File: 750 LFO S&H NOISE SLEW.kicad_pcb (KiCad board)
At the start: 2 copper layers, 65 x 106.5 mm, 239 parts, among them J1 PJ301BM, J10 PJ301BM, J11 PJ301BM, J2 PJ301BM, J3 PJ301BM, J4 PJ301BM, J5 JACK_MONO_SW, J6 PJ301BM, J7 JACK_MONO_SW, J8 PJ301BM, J9 PJ301BM, P1 CONN_01X03, P3 CONN_02X05, Q1 MMBT3904, Q10 MMBT3904, Q11 J112, Q12 MMBT3906, Q13 J112, Q14 J112, Q15 MMBT3904, Q16 MMBT3904, Q2 MMBT3904, Q3 2N7002, Q4 2N7002, Q5 MBT3946DW, Q6 MBT3946DW, Q7 MMBT3904, Q8 MMBT3904, Q9 MMBT3904, SW1 KS-01Q, SW2 KS-01Q, SW3 SPDT, U1 LM13700, U10 TL072-, U11 TL072-, U12 MAX9945, U13 DG409, U14 DG409, U15 TS321, U2 TL072-, U3 TL072-, U4 TL072-, U5 TL072-, U6 CD40106, U7 CD4027, U8 CD4027, U9 TL072-

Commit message: notes
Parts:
- R25: value 10K -> 22K
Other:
- board text removed: "SN#"
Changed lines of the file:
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@@
     (links 501)
     (no_connects 0)
-    (area 59.924999 24.924999 125.075001 131.575001)
+    (area 56.936905 22.45604 128.313095 132.325001)
     (thickness 1.6)
     (drawings 942)
@@
     (35 F.Paste user)
     (36 B.SilkS user)
-    (37 F.SilkS user)
+    (37 F.SilkS user hide)
     (38 B.Mask user)
     (39 F.Mask user)
@@
     (pad_to_mask_clearance 0.01)
     (aux_axis_origin 0 0)
-    (visible_elements 7FFFF77F)
+    (visible_elements 7FFFB7FF)
     (pcbplotparams
       (layerselection 0x010f0_80000001)
@@
       (effects (font (size 0.6096 0.6096) (thickness 0.1524)) (justify mirror))
     )
-    (fp_text value 2N7002 (at 1.016 -2.286 90) (layer B.SilkS) hide
+    (fp_text value 2N7002 (at -1.25 -0.5 90) (layer B.SilkS) hide
       (effects (font (size 0.8128 0.8128) (thickness 0.1524)) (justify mirror))
     )
@@
       (effects (font (size 0.6096 0.6096) (thickness 0.1524)) (justify mirror))
     )
-    (fp_text value 2N7002 (at 1.016 -2.286 90) (layer B.SilkS) hide
+    (fp_text value 2N7002 (at 1.2 0.05 90) (layer B.SilkS) hide
       (effects (font (size 0.8128 0.8128) (thickness 0.1524)) (justify mirror))
     )
@@
       (effects (font (size 0.6096 0.6096) (thickness 0.1524)) (justify mirror))
     )
-    (fp_text value 1N4148 (at 0 -1.905 90) (layer B.SilkS) hide
+    (fp_text value 1N4148 (at 0.15 -0.05 90) (layer B.SilkS) hide
       (effects (font (size 1 1) (thickness 0.15)) (justify mirror))
     )
@@
       (effects (font (size 0.6096 0.6096) (thickness 0.1524)) (justify mirror))
     )
-    (fp_text value 10K (at 0 0 270) (layer B.SilkS) hide
+    (fp_text value 22K (at 0 0 270) (layer B.SilkS) hide
       (effects (font (size 0.508 0.4572) (thickness 0.1143)) (justify mirror))
     )
@@
     (at 75.5 45.5 180)
     (attr smd)
-    (fp_text reference R99 (at -3 -0.75 180) (layer B.SilkS)
+    (fp_text reference R99 (at -0.1 -1.4 180) (layer B.SilkS)
       (effects (font (size 0.6096 0.6096) (thickness 0.1524)) (justify mirror))
     )
@@
     )
   )
-  (gr_text SN# (at 113.5 129.9) (layer B.SilkS)
-    (effects (font (size 1 1) (thickness 0.15)) (justify mirror))
-  )
+  (gr_line (start 63.45 66.9) (end 63.45 66.9) (angle 90) (layer B.SilkS) (width 5))
   (gr_line (start 109.4 128.3) (end 106.4 128.3) (angle 90) (layer B.SilkS) (width 5))
   (gr_text 850 (at 92.4 128.4) (layer B.SilkS)
@@
   (gr_line (start 68.000117 32.50286) (end 68.000117 34.50286) (layer Eco2.User) (width 0.1))
   (gr_text -12V (at 116.1 111.7) (layer B.SilkS)
-    (effects (font (size 1 1) (thickness 0.1524)) (justify mirror))
+    (effects (font (size 1.2 1.2) (thickness 0.25)) (justify mirror))
   )
   (gr_line (start 123.75 109.75) (end 116.25 109.75) (angle 90) (layer B.SilkS) (width 2))

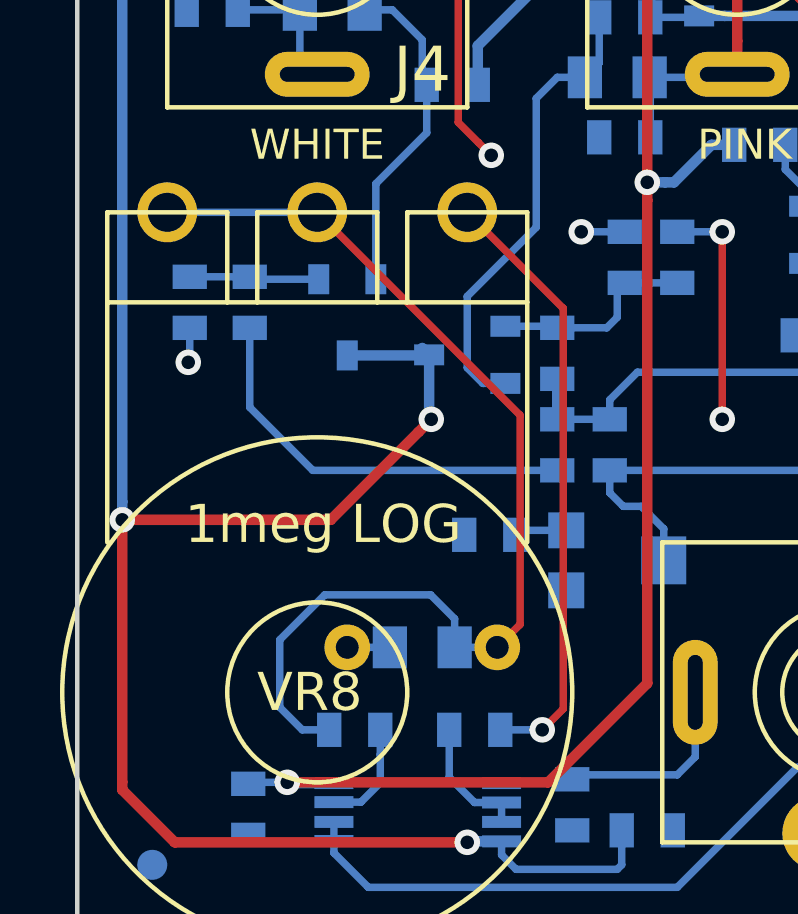
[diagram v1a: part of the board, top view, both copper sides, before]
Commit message: commit before adding voltage referencd for LFO
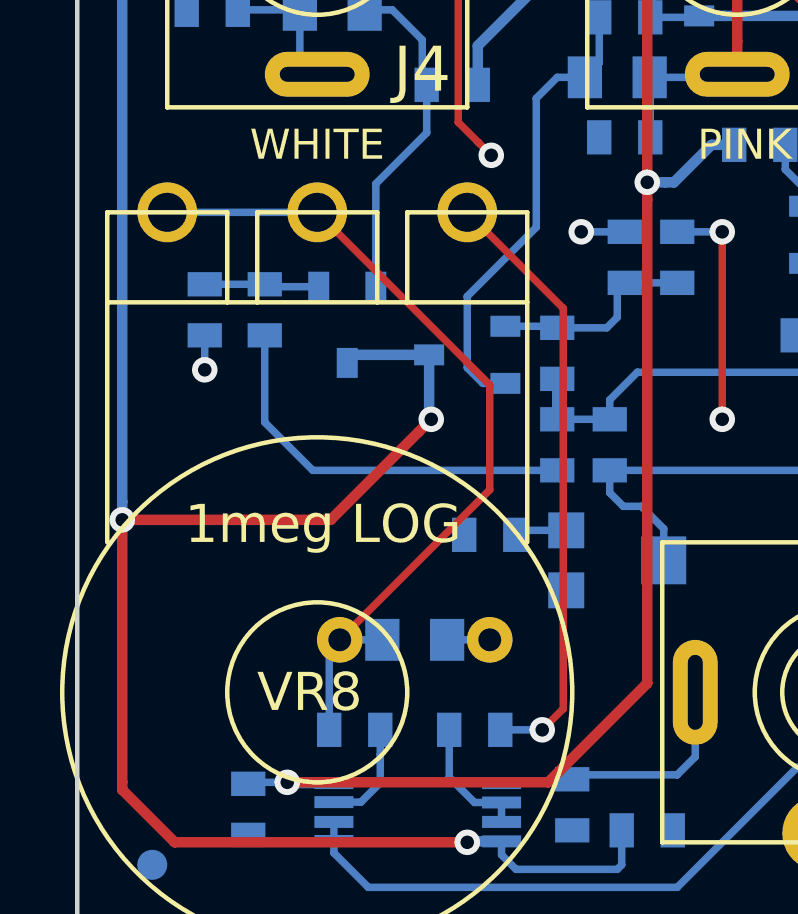
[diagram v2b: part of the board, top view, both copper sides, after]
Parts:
- moved R26 0.56 mm to (66.2, 110.8)
- moved R29 0.56 mm to (64.2, 110.8)
- moved C44 0.35 mm to (71.2, 121.8), turned to 0 degrees
- moved Q9 0.25 mm to (69.0, 111.2)
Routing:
- net Net-(C44-Pad1): track 36.0 -> 28.3 mm
- net Net-(Q9-Pad1): track 4.57 -> 4.07 mm
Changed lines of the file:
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@@
     (thickness 1.6)
     (drawings 942)
-    (tracks 1971)
+    (tracks 1964)
     (zones 0)
     (modules 239)
@@
   )
   (module MyModules:SOT23-132-JRL (layer B.Cu)
-    (at 69 111)
+    (at 69 111.25)
     (tags SOT23)
     (fp_text reference Q9 (at 1.99898 0.09906 270) (layer B.SilkS)
@@
   )
   (module MyModules:SM0603-R-JRL (layer B.Cu)
-    (at 65.75 110.5 90)
+    (at 66.25 110.75 90)
     (attr smd)
     (fp_text reference R26 (at 2 0 180) (layer B.SilkS)
@@
   )
   (module MyModules:SM0603-R-JRL (layer B.Cu)
-    (at 63.75 110.5 270)
+    (at 64.25 110.75 270)
     (attr smd)
     (fp_text reference R29 (at 0 1.4 270) (layer B.SilkS)
@@
   )
   (module MyModules:CAP-5MM-BOX-0805-COMBO (layer B.Cu)
-    (at 71.5 122 180)
-    (fp_text reference C44 (at 4.4 0 270) (layer B.SilkS)
+    (at 71.25 121.75)
+    (fp_text reference C44 (at 4.4 0 90) (layer B.SilkS)
       (effects (font (size 0.8128 0.8128) (thickness 0.1524)) (justify mirror))
     )
-    (fp_text value 470n (at 1.6 2.6 180) (layer B.Fab) hide
+    (fp_text value 470n (at 1.6 2.6) (layer B.Fab) hide
       (effects (font (size 1 1) (thickness 0.15)) (justify mirror))
     )
@@
     (fp_line (start -1.75 0.75) (end -1.75 -0.75) (layer B.SilkS) (width 0.15))
     (fp_line (start 1.75 0.75) (end 1.75 -0.75) (layer B.SilkS) (width 0.15))
-    (pad 1 thru_hole circle (at -2.5 0 180) (size 1.524 1.524) (drill 0.762) (layers *.Cu *.Mask B.SilkS)
+    (pad 1 thru_hole circle (at -2.5 0) (size 1.524 1.524) (drill 0.762) (layers *.Cu *.Mask B.SilkS)
       (net 35 "Net-(C44-Pad1)"))
-    (pad 2 thru_hole circle (at 2.5 0 180) (size 1.524 1.524) (drill 0.762) (layers *.Cu *.Mask B.SilkS)
+    (pad 2 thru_hole circle (at 2.5 0) (size 1.524 1.524) (drill 0.762) (layers *.Cu *.Mask B.SilkS)
       (net 1 GND))
-    (pad 1 smd rect (at -1.0795 0 180) (size 1.143 1.397) (layers B.Cu B.Paste B.Mask)
+    (pad 1 smd rect (at -1.0795 0) (size 1.143 1.397) (layers B.Cu B.Paste B.Mask)
       (net 35 "Net-(C44-Pad1)"))
-    (pad 2 smd rect (at 1.0795 0 180) (size 1.143 1.397) (layers B.Cu B.Paste B.Mask)
+    (pad 2 smd rect (at 1.0795 0) (size 1.143 1.397) (layers B.Cu B.Paste B.Mask)
       (net 1 GND))
   )
@@
   (gr_line (start 125 25) (end 125 131.5) (angle 90) (layer Edge.Cuts) (width 0.15))
   (gr_line (start 60 25) (end 125 25) (angle 90) (layer Edge.Cuts) (width 0.15))
+  (segment (start 64.25 111.6009) (end 64.25 112.75) (width 0.25) (layer B.Cu) (net 1))
+  (via (at 64.25 112.75) (size 0.85) (drill 0.45) (layers F.Cu B.Cu) (net 1))
+  (segment (start 72.3295 121.75) (end 73.75 121.75) (width 0.25) (layer B.Cu) (net 1))
   (segment (start 93.5 117.3) (end 90.7 114.5) (width 0.25) (layer F.Cu) (net 1))
   (segment (start 90.7 114.5) (end 90.1 114.5) (width 0.25) (layer F.Cu) (net 1))
@@
   (segment (start 96.1509 115.6509) (end 95.4 114.9) (width 0.25) (layer B.Cu) (net 1))
   (via (at 95.4 114.9) (size 0.85) (drill 0.45) (layers F.Cu B.Cu) (net 1))
-  (segment (start 63.75 111.3509) (end 63.75 112.45) (width 0.25) (layer B.Cu) (net 1))
-  (segment (start 63.75 112.45) (end 63.7 112.5) (width 0.25) (layer B.Cu) (net 1))
-  (via (at 63.7 112.5) (size 0.85) (drill 0.45) (layers F.Cu B.Cu) (net 1))
   (segment (start 73.375001 105.175001) (end 73.8 105.6) (width 0.25) (layer F.Cu) (net 1))
   (segment (start 72.7 104.5) (end 73.375001 105.175001) (width 0.25) (layer F.Cu) (net 1))
@@
   (segment (start 114.5475 39.2975) (end 114 38.75) (width 0.25) (layer B.Cu) (net 1))
   (via (at 114 38.75) (size 0.85) (drill 0.45) (layers F.Cu B.Cu) (net 1))
-  (segment (start 70.4205 122) (end 69 122) (width 0.25) (layer B.Cu) (net 1))
   (segment (start 110.15158 28.075) (end 111.775 28.075) (width 0.25) (layer B.Cu) (net 1))
   (segment (start 111.775 28.075) (end 111.8 28.1) (width 0.25) (layer B.Cu) (net 1))
@@
   (segment (start 90.05 105.1991) (end 90.05 102.5991) (width 0.25) (layer B.Cu) (net 3))
   (segment (start 90.05 102.5991) (end 90.0009 102.55) (width 0.25) (layer B.Cu) (net 3))
+  (segment (start 69 112.52) (end 69.27 112.25) (width 0.35) (layer B.Cu) (net 4))
+  (segment (start 69.27 112.25) (end 71.73 112.25) (width 0.35) (layer B.Cu) (net 4))
   (segment (start 69.2 89.699998) (end 64.050002 89.699998) (width 0.35) (layer B.Cu) (net 4))
   (segment (start 64.050002 89.699998) (end 61.5 92.25) (width 0.35) (layer B.Cu) (net 4))
@@
   (segment (start 61.5 126.5) (end 61.5 117.75) (width 0.35) (layer F.Cu) (net 4))
   (via (at 61.5 117.75) (size 0.85) (drill 0.45) (layers F.Cu B.Cu) (net 4))
-  (segment (start 69 112.27) (end 71.71 112.27) (width 0.35) (layer B.Cu) (net 4))
-  (segment (start 71.71 112.27) (end 71.73 112.25) (width 0.35) (layer B.Cu) (net 4))
   (segment (start 95.7 83) (end 95.7 75.3) (width 0.8) (layer F.Cu) (net 4))
   (segment (start 95.7 75.3) (end 99.9 71.1) (width 0.8) (layer F.Cu) (net 4))
@@
   (segment (start 118.5 88.7) (end 118.5 85.7) (width 0.8) (layer F.Cu) (net 4))
   (via (at 118.5 85.7) (size 0.85) (drill 0.45) (layers F.Cu B.Cu) (net 4))
-  (segment (start 71.5 112.02) (end 71.73 112.25) (width 0.35) (layer B.Cu) (net 4))
   (segment (start 88.3991 106.9) (end 88.3991 107.75) (width 0.35) (layer B.Cu) (net 4))
   (segment (start 100.45 28.875) (end 99.35 28.875) (width 0.35) (layer B.Cu) (net 4))
@@
   (segment (start 80 109.8509) (end 78.25 109.8509) (width 0.25) (layer B.Cu) (net 12))
   (segment (start 76 116.1009) (end 67.8509 116.1009) (width 0.25) (layer B.Cu) (net 13))
-  (segment (start 67.8509 116.1009) (end 65.75 114) (width 0.25) (layer B.Cu) (net 13))
-  (segment (start 65.75 114) (end 65.75 111.3509) (width 0.25) (layer B.Cu) (net 13))
+  (segment (start 67.8509 116.1009) (end 66.25 114.5) (width 0.25) (layer B.Cu) (net 13))
+  (segment (start 66.25 114.5) (end 66.25 111.6009) (width 0.25) (layer B.Cu) (net 13))
   (segment (start 77.75 114.3991) (end 77.75 113.75) (width 0.25) (layer B.Cu) (net 14))
   (segment (start 77.75 113.75) (end 78.6696 112.8304) (width 0.25) (layer B.Cu) (net 14))
@@
   (segment (start 69.9525 106.5475) (end 71.6491 104.8509) (width 0.25) (layer B.Cu) (net 20))
   (segment (start 71.6491 104.8509) (end 71.6491 103.25) (width 0.25) (layer B.Cu) (net 20))
-  (segment (start 69.9525 109.73) (end 69.9525 106.5475) (width 0.25) (layer B.Cu) (net 20))
+  (segment (start 69.9525 109.98) (end 69.9525 106.5475) (width 0.25) (layer B.Cu) (net 20) (status 10))
   (segment (start 97.5 101.98) (end 96.89948 101.98) (width 0.25) (layer B.Cu) (net 21))
   (segment (start 96.89948 101.98) (end 94.87948 104) (width 0.25) (layer B.Cu) (net 21))
@@
   (segment (start 98.75 50.6009) (end 100.5 50.6009) (width 0.25) (layer B.Cu) (net 34))
   (segment (start 97 50.6009) (end 98.75 50.6009) (width 0.25) (layer B.Cu) (net 34))
-  (segment (start 74 122) (end 74.761999 121.238001) (width 0.25) (layer F.Cu) (net 35))
-  (segment (start 74.761999 121.238001) (end 74.761999 114.261999) (width 0.25) (layer F.Cu) (net 35))
-  (segment (start 74.761999 114.261999) (end 68 107.5) (width 0.25) (layer F.Cu) (net 35))
+  (segment (start 68.75 121.75) (end 73.75 116.75) (width 0.25) (layer F.Cu) (net 35))
+  (segment (start 73.75 116.75) (end 73.75 113.25) (width 0.25) (layer F.Cu) (net 35))
+  (segment (start 73.75 113.25) (end 68 107.5) (width 0.25) (layer F.Cu) (net 35))
+  (segment (start 68.3991 124.75) (end 68.3991 122.1009) (width 0.25) (layer B.Cu) (net 35))
+  (segment (start 68.3991 122.1009) (end 68.75 121.75) (width 0.25) (layer B.Cu) (net 35))
+  (segment (start 70.1705 121.75) (end 68.75 121.75) (width 0.25) (layer B.Cu) (net 35))
   (segment (start 68 107.5) (end 63 107.5) (width 0.25) (layer B.Cu) (net 35))
-  (segment (start 72.5795 122) (end 74 122) (width 0.25) (layer B.Cu) (net 35))
-  (segment (start 72.5795 122) (end 72.5795 121.0515) (width 0.25) (layer B.Cu) (net 35))
-  (segment (start 67.5 124.75) (end 68.3991 124.75) (width 0.25) (layer B.Cu) (net 35))
-  (segment (start 72.5795 121.0515) (end 71.778 120.25) (width 0.25) (layer B.Cu) (net 35))
-  (segment (start 71.778 120.25) (end 68.25 120.25) (width 0.25) (layer B.Cu) (net 35))
-  (segment (start 68.25 120.25) (end 66.75 121.75) (width 0.25) (layer B.Cu) (net 35))
-  (segment (start 66.75 121.75) (end 66.75 124) (width 0.25) (layer B.Cu) (net 35))
-  (segment (start 66.75 124) (end 67.5 124.75) (width 0.25) (layer B.Cu) (net 35))
   (segment (start 94.4446 107.9) (end 94.4 107.8554) (width 0.25) (layer B.Cu) (net 36))
   (segment (start 94.4 107.8554) (end 94.4 106.4991) (width 0.25) (layer B.Cu) (net 36))
@@
   (segment (start 91.3991 81.2009) (end 91.3991 82.25) (width 0.25) (layer B.Cu) (net 78))
   (segment (start 91.6023 79.79756) (end 91.6023 80.9977) (width 0.25) (layer B.Cu) (net 78))
-  (segment (start 68.0475 109.73) (end 65.8309 109.73) (width 0.25) (layer B.Cu) (net 79))
-  (segment (start 65.8309 109.73) (end 65.75 109.6491) (width 0.25) (layer B.Cu) (net 79))
-  (segment (start 65.9191 109.48) (end 65.75 109.6491) (width 0.25) (layer B.Cu) (net 79) (status 30))
-  (segment (start 63.75 109.6491) (end 65.75 109.6491) (width 0.25) (layer B.Cu) (net 79) (status 20))
+  (segment (start 68.0475 109.98) (end 66.3309 109.98) (width 0.25) (layer B.Cu) (net 79) (status 10))
+  (segment (start 66.3309 109.98) (end 66.25 109.8991) (width 0.25) (layer B.Cu) (net 79) (status 30))
+  (segment (start 66.4191 109.73) (end 66.25 109.8991) (width 0.25) (layer B.Cu) (net 79) (status 30))
+  (segment (start 64.25 109.8991) (end 66.25 109.8991) (width 0.25) (layer B.Cu) (net 79) (status 10))
   (segment (start 92.25 70.48) (end 92.43 70.3) (width 0.25) (layer B.Cu) (net 80))
   (segment (start 92.43 70.3) (end 93.8009 70.3) (width 0.25) (layer B.Cu) (net 80))
